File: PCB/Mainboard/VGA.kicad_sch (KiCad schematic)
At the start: 2 parts, among them U51 CHIPS65535

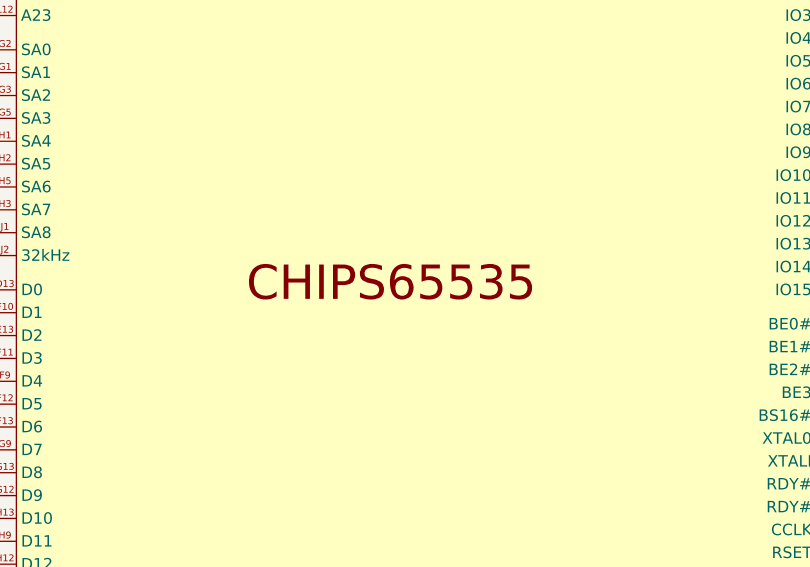
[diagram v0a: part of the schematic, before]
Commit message: Add files via upload
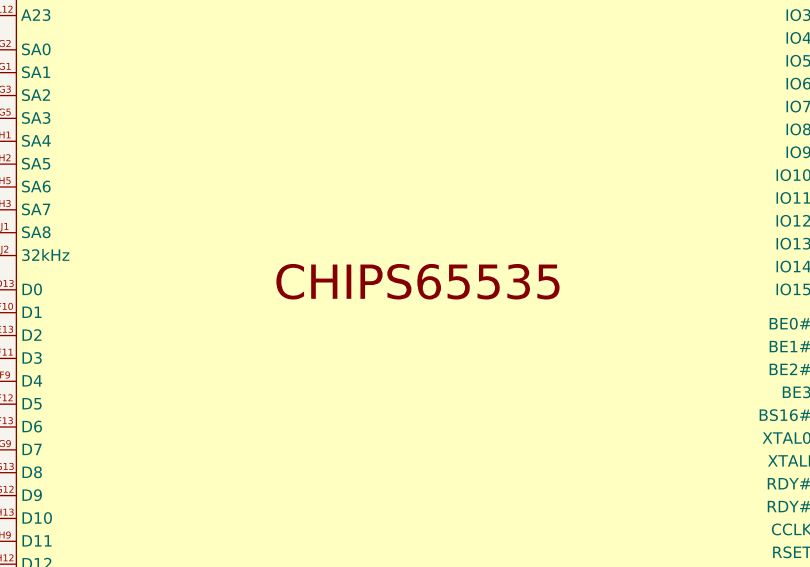
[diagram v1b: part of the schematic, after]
